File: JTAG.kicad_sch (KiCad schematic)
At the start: 21 parts, among them U1 XC7Z020-1CLG400I__, U4 ATSHA204A-SSHCZ-T, U7 S25FL128SAGMFI000

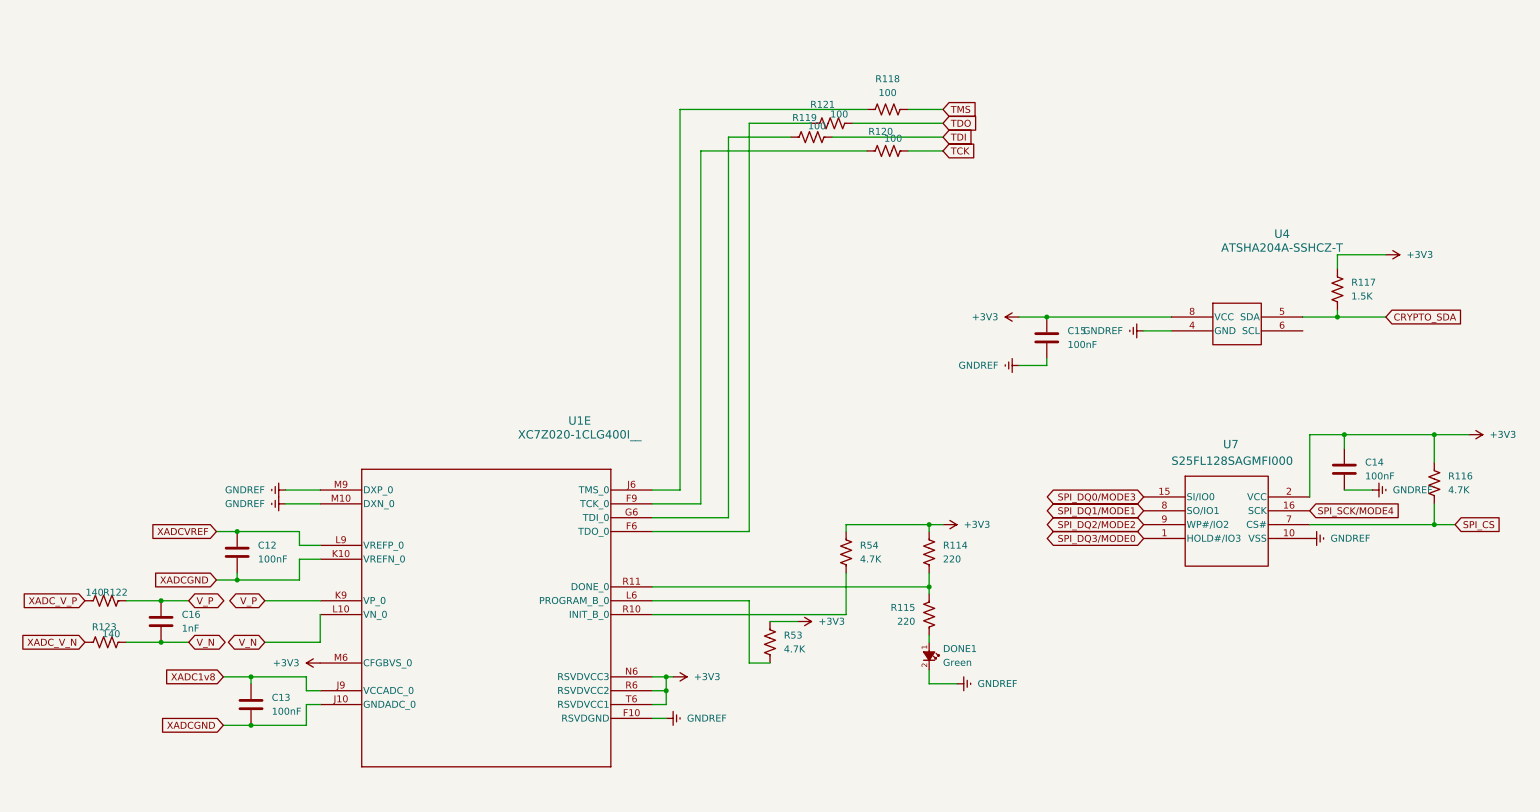
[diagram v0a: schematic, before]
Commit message: ready for manufacturing
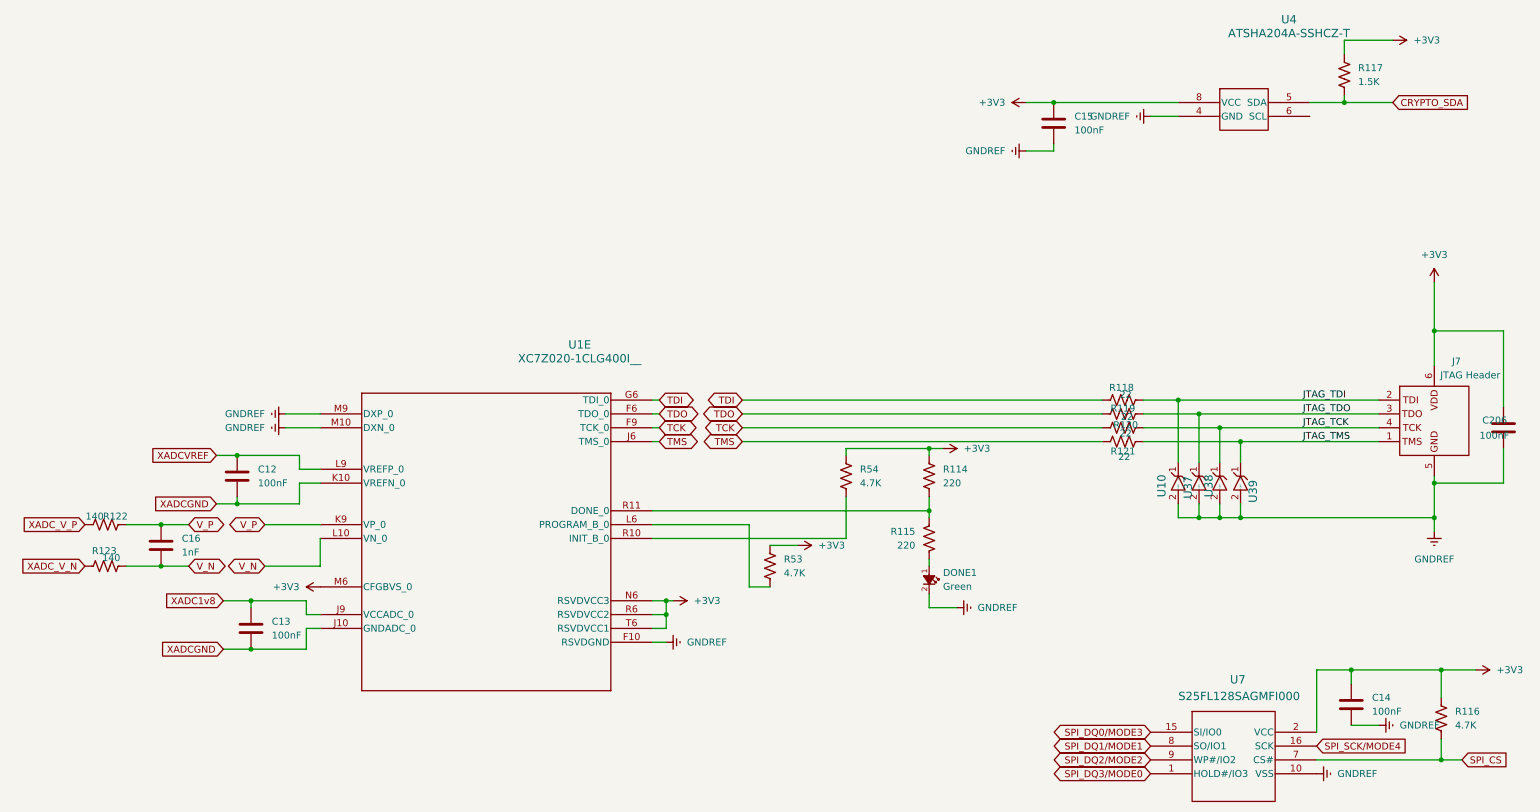
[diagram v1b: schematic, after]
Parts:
- added C206: 100nF, footprints:C_0201_0603Metric, symbol Device:C
- added J7: JTAG Header, footprints:PinHeader_1x06_P2.54mm_Vertical, symbol Connector:Conn_01x06_Pin
- added U10, U37, U38, U39: TPD1E05U06DPYR, footprints:DIO_TPD1E05U06DPYR, symbol TPD1E05U06DPYR:TPD1E05U06DPYR
- C12, C13, C15: LCSC PN c1525 -> c307380
- C14: footprint footprints:C_0402 -> footprints:C_0201_0603Metric; LCSC PN c1525 -> c307380
- C16: footprint footprints:C_0201_0603Metric -> footprints:C_0402; LCSC PN c14442 -> C77018
- R116, R53, R54: footprint footprints:R_0402 -> footprints:R_0201_0603Metric; LCSC PN C105871 -> C138135
- R118, R119, R120, R121: value 100 -> 22; footprint footprints:R_0402 -> footprints:R_0201_0603Metric; LCSC PN C106232 -> C270355
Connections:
- net +3V3: now also C206.1, J7.6 (VDD)
- net GNDREF: now also U7.3 (RESET#/RFU), C206.2, J7.5 (GND), U10.2 (GND), U37.2 (GND), U38.2 (GND), U39.2 (GND)
- net TCK: now also R120.1, U1.F9 (TCK_0); no longer R120.2
- net TDI: now also R118.1, U1.G6 (TDI_0); no longer R119.2
- net TDO: now also R119.1, U1.F6 (TDO_0); no longer R121.2
- net TMS: now also R121.1, U1.J6 (TMS_0); no longer R118.2
- new net JTAG_TCK: J7.4 (TCK), R120.2, U38.1 (I/O)
- new net JTAG_TDI: J7.2 (TDI), R118.2, U10.1 (I/O)
- new net JTAG_TDO: J7.3 (TDO), R119.2, U37.1 (I/O)
- new net JTAG_TMS: J7.1 (TMS), R121.2, U39.1 (I/O)
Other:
- moved on the sheet: C12, C13, C14, C15, C16, DONE1, R114, R115, R116, R117, R122, R123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
